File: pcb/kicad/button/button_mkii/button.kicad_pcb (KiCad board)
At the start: 2 copper layers, 160 parts, among them J1 SWD, J2 RESET_CONN, J3 ADC_OUT, U1 STBlueNRG-1, U2 TLV1117LV-3V, Y1 Xtal 32.768kHz, Y2 XTAL 32MHz

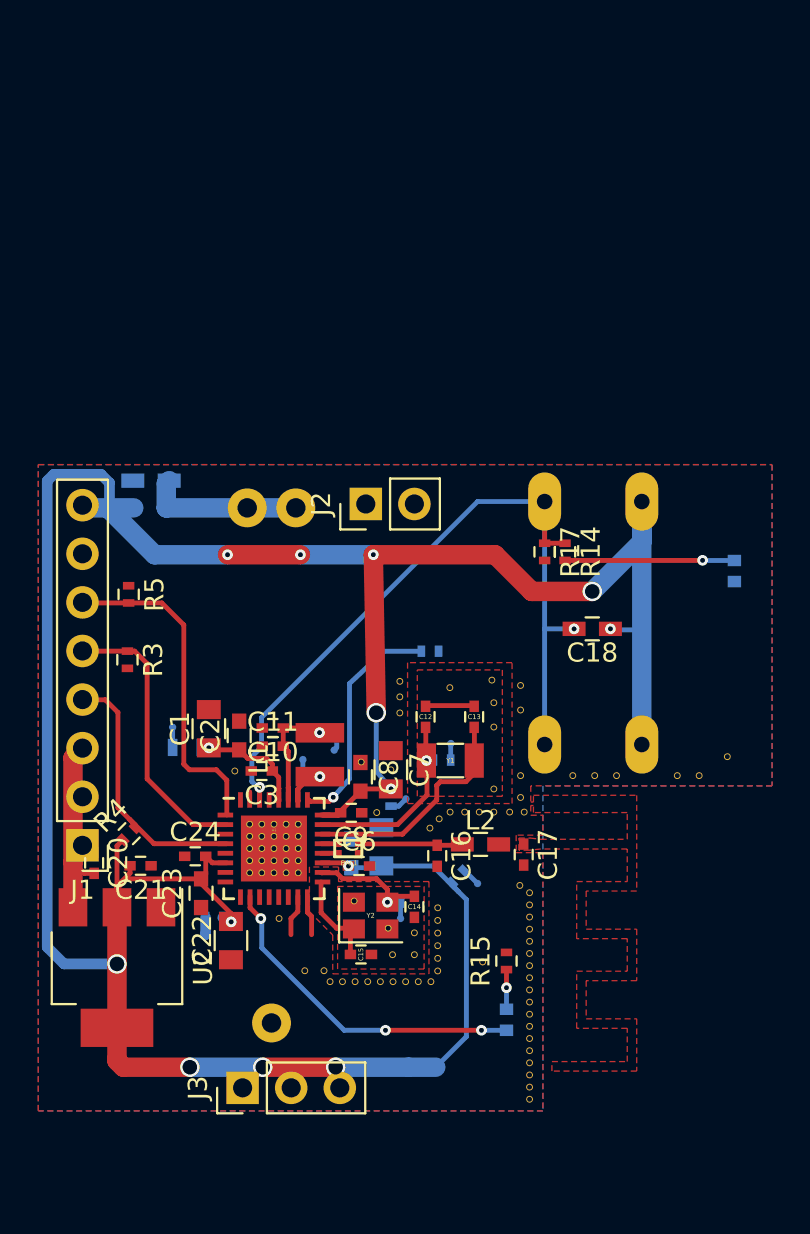
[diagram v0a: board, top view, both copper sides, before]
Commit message: rev3.1
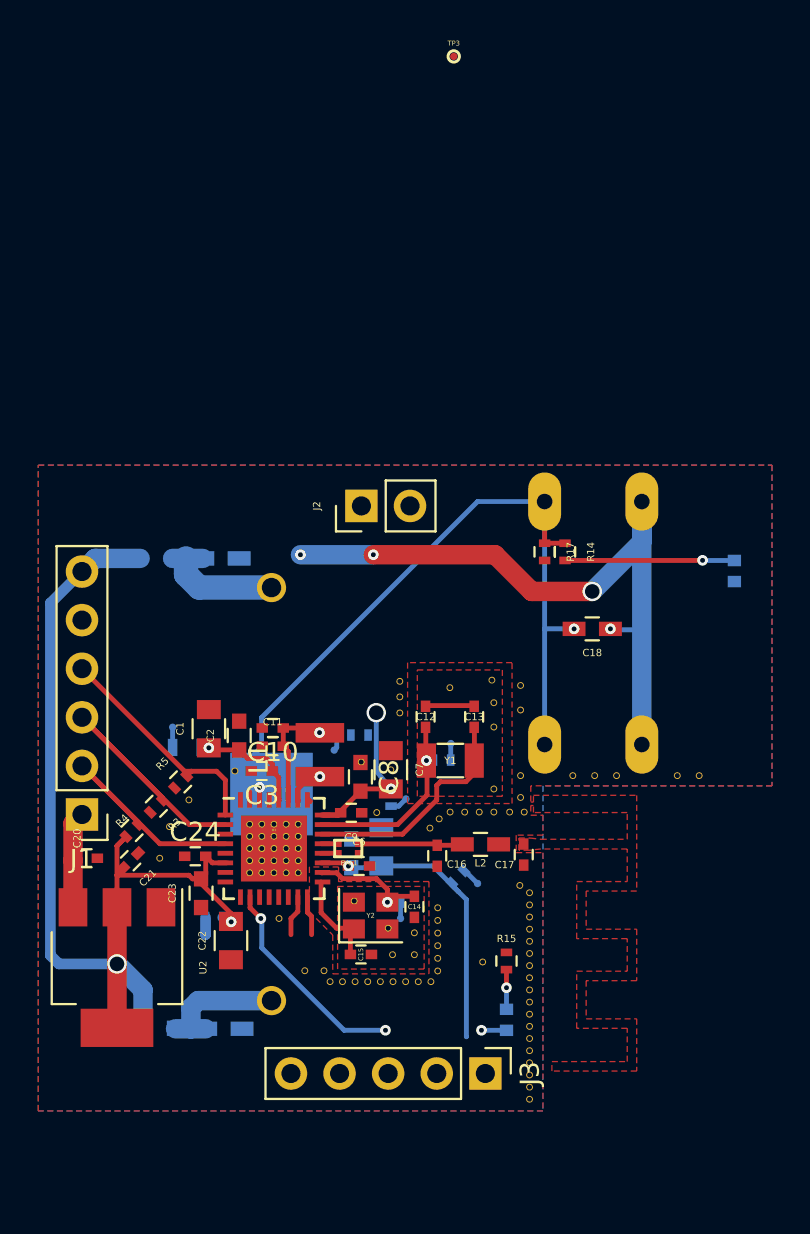
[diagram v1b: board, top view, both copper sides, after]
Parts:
- added C25: 1uF, Capacitors_SMD:C_0603_HandSoldering, B.Cu at (119.0, 113.7)
- added D4: Power thru Battery, Diodes_SMD:D_0603, B.Cu at (115.5, 113.7)
- added REF**: Via_Stitch_Dia0.356mm_Drill0.254mm, Miscellaneous:Via_Stitch_Dia0.356mm_Drill0.254mm, F.Cu at (117.2, 101.7)
- added REF**: Via_Stitch_Dia0.356mm_Drill0.254mm, Miscellaneous:Via_Stitch_Dia0.356mm_Drill0.254mm, F.Cu at (116.2, 103.1)
- added TP3: VBATT2, Miscellaneous:Measurement_Point_Round-SMD-tiniest, F.Cu at (131.1, 62.9)
- BT1: value Battery_Cell -> Battery; footprint Batteries:CoinCell_holder_1060x630 -> Batteries:batt_holder3035
- J1: value SWD -> CONN_01X06; footprint Pin_Headers:Pin_Header_Straight_1x08_Pitch2.54mm -> Pin_Headers:Pin_Header_Straight_1x06_Pitch2.54mm
- J3: value ADC_OUT -> CONN_01X05; footprint Pin_Headers:Pin_Header_Straight_1x03_Pitch2.54mm -> Pin_Headers:Pin_Header_Straight_1x05_Pitch2.54mm
- moved REF** 30.1 mm to (115.7, 104.8)
- moved J3 12.7 mm to (132.7, 116.0), turned to 270 degrees
- moved R5 10.2 mm to (116.8, 100.8), turned to 45 degrees
- moved R3 7.81 mm to (115.5, 102.1), turned to 225 degrees
- moved R13 5.72 mm to (126.1, 98.3)
- moved C19 5.47 mm to (118.9, 89.1), turned to 0 degrees
- moved D3 2.66 mm to (115.5, 89.1)
- moved J1 1.61 mm to (111.6, 102.5)
- moved BT1 1.50 mm to (121.5, 101.4)
- moved C21 0.59 mm to (114.2, 104.9), turned to 225 degrees
- moved C20 0.45 mm to (111.9, 104.8), turned to 180 degrees
- moved J2 0.25 mm to (126.2, 86.4)
- moved R4 0.22 mm to (114.2, 103.3)
- renumbered TP3 to VBATT2
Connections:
- BT1 pad 2: Net-(BT1-Pad1) -> GND
- J1 pad 2: Net-(J1-Pad2) -> DIO7
- J1 pad 3: Net-(J1-Pad3) -> DIO9
- J1 pad 4: DIO7 -> DIO10
- J1 pad 5: DIO9 -> GND
- J1 pad 6: DIO10 -> +3V3
- J3 pad 2: ADC1 -> ADC2
- J3 pad 3: ADC2 -> ADC1
- R13 pad 1: GND -> +3V3
- U1 pad 11: Net-(J1-Pad3) -> Net-(J3-Pad5)
- U1 pad 12: Net-(J1-Pad2) -> Net-(J3-Pad4)
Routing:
- net +3V3: track 173.6 -> 128.8 mm, vias 13 -> 9
- net GND: track 19.3 -> 40.3 mm, vias 0 -> 1
- net /DIO12_BUTTON: track 42.4 -> 22.4 mm, vias 2 -> 1
- net Net-(J2-Pad1): track 12.3 -> 0.32 mm, vias 1 -> 0
- net Net-(J1-Pad3): track 6.15 -> 0.00 mm
- net Net-(BT1-Pad1): track 8.26 -> 14.2 mm
- net DIO10: track 17.5 -> 12.1 mm
- net /DIO2_LED: track 17.6 -> 12.5 mm
- net Net-(C20-Pad2): track 3.71 -> 5.05 mm
- net DIO9: track 14.8 -> 15.9 mm
- net Net-(R11-Pad2): track 0.90 -> 0.00 mm
- net DIO7: track 14.1 -> 13.5 mm

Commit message: rev3.1_layout
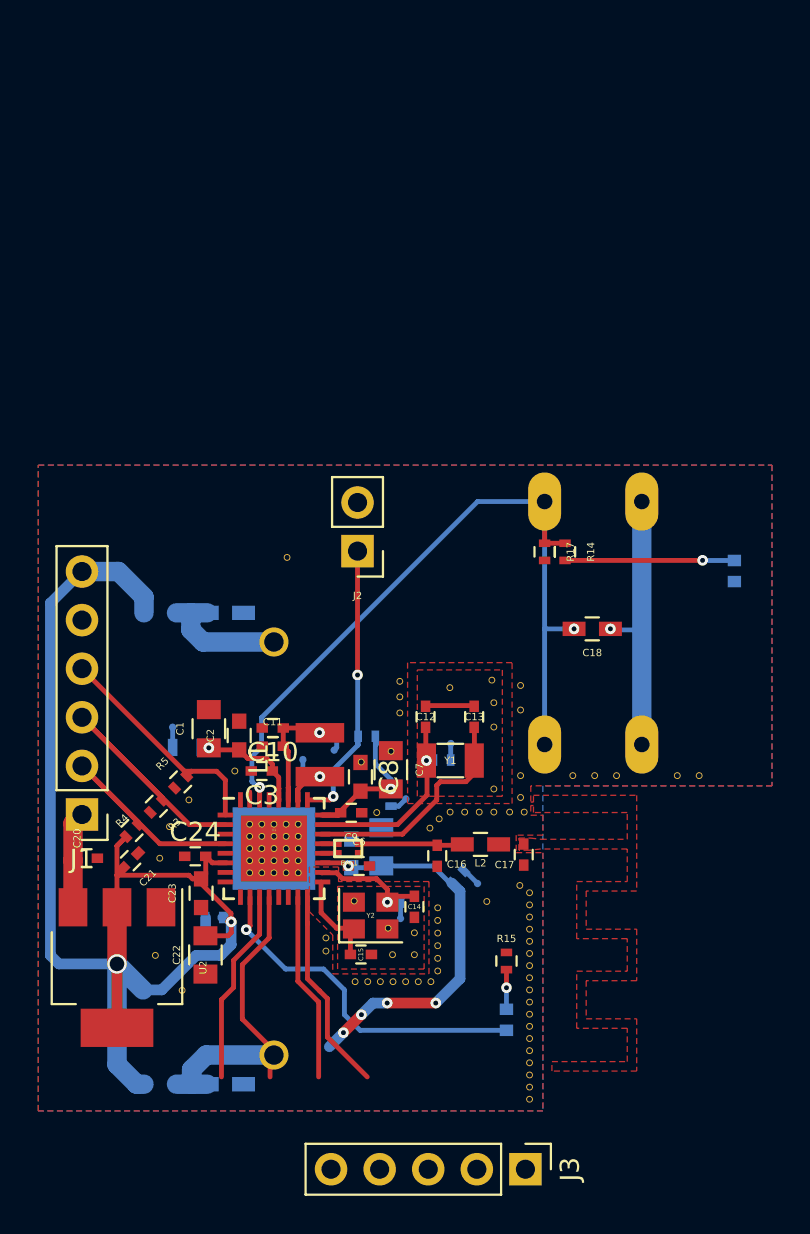
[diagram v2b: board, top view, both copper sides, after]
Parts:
- removed TP3: VBATT2, Miscellaneous:Measurement_Point_Round-SMD-tiniest
- BT1: value Battery -> Battery_cc3035; footprint Batteries:batt_holder3035 -> batt_holder3035
- moved REF** 22.3 mm to (122.4, 89.1)
- moved REF** 8.63 mm to (132.8, 107.0)
- moved REF** 8.29 mm to (124.4, 108.9)
- moved REF** 6.75 mm to (115.5, 109.9)
- moved REF** 6.50 mm to (116.9, 111.7)
- moved J3 5.42 mm to (134.8, 121.0)
- moved D4 2.93 mm to (115.7, 116.6)
- moved C25 2.90 mm to (119.1, 116.6)
- moved C19 2.85 mm to (119.1, 91.9)
- moved D3 2.85 mm to (115.7, 91.9)
- moved BT1 2.85 mm to (121.7, 104.3)
- moved J2 2.37 mm to (126.0, 88.7), turned to 180 degrees
- moved C22 1.53 mm to (118.1, 109.8)
- moved REF** 1.03 mm to (124.4, 109.6)
- moved REF** 0.97 mm to (127.8, 99.2)
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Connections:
- BT1 pad 2: GND -> Net-(BT1-Pad2)
- C25 pad 1: Net-(BT1-Pad1) -> Net-(BT1-Pad2)
- D4 pad 2: Net-(BT1-Pad1) -> Net-(BT1-Pad2)
- U2 pad 4: (no net) -> +3V3
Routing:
- net GND: track 40.3 -> 19.3 mm, vias 1 -> 0
- net /DIO12_BUTTON: track 22.4 -> 42.4 mm, vias 1 -> 2
- net Net-(J2-Pad1): track 0.32 -> 15.3 mm, vias 0 -> 2
- net Net-(BT1-Pad2): track 0.00 -> 10.8 mm
- net Net-(J3-Pad5): track 0.00 -> 10.2 mm
- net ADC2: track 2.13 -> 10.7 mm
- net ADC1: track 2.19 -> 9.85 mm
- net Net-(BT1-Pad1): track 14.2 -> 7.10 mm
- net Net-(J3-Pad4): track 0.00 -> 6.96 mm
- net /DIO2_LED: track 12.5 -> 18.3 mm, vias 3 -> 1
- net +3V3: track 128.8 -> 127.6 mm
- net Net-(R11-Pad2): track 0.00 -> 0.90 mm
